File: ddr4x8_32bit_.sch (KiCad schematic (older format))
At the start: 71 parts

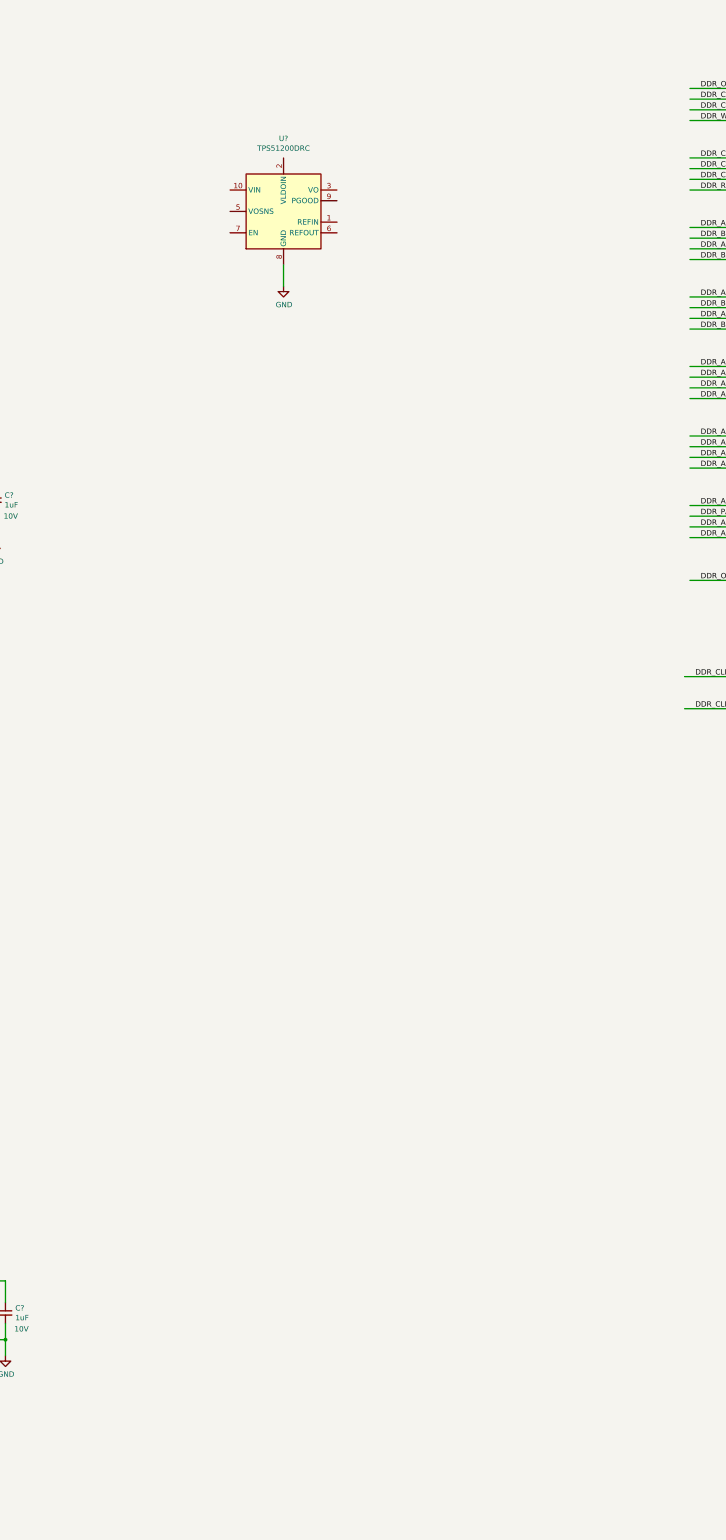
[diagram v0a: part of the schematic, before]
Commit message: Schematic capture update.
Schematic capture update(DDR).
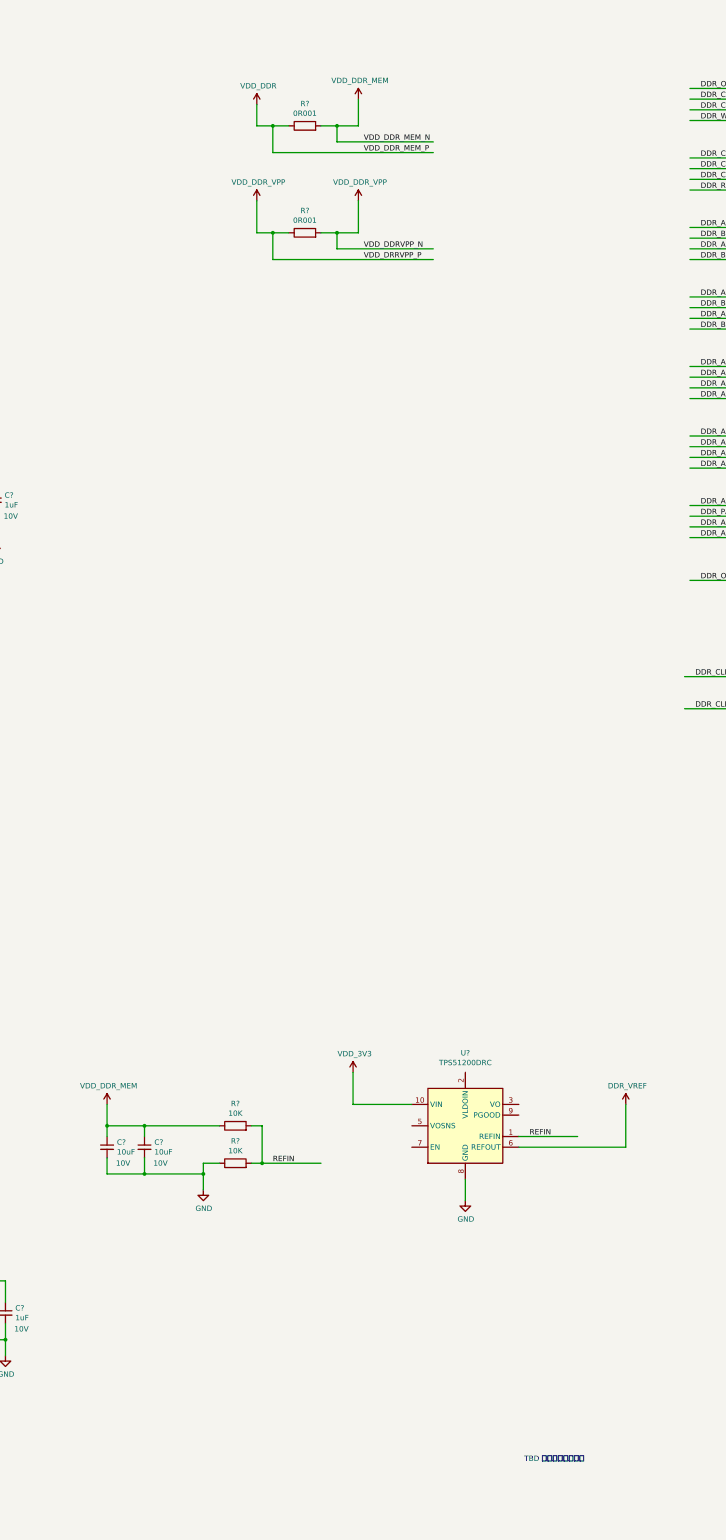
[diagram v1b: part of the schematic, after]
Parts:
- added C? (x2): 10uF, symbol Device:C_Small
- added R? (x2): 0R001, symbol Device:R
- added R? (x2): 10K, symbol Device:R
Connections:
- net labels added: REFIN, VDD_3V3, VDD_DDR, VDD_DDRVPP_N, VDD_DDR_MEM_N, VDD_DDR_MEM_P, VDD_DRRVPP_P
- wire segments 719 -> 760
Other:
- note added: "TBD レイアウトノート"
- moved on the sheet: U?
